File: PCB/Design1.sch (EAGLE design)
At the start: 23 parts, among them J1 FTDI_DEVICE, U1 ATMEGA2560AU

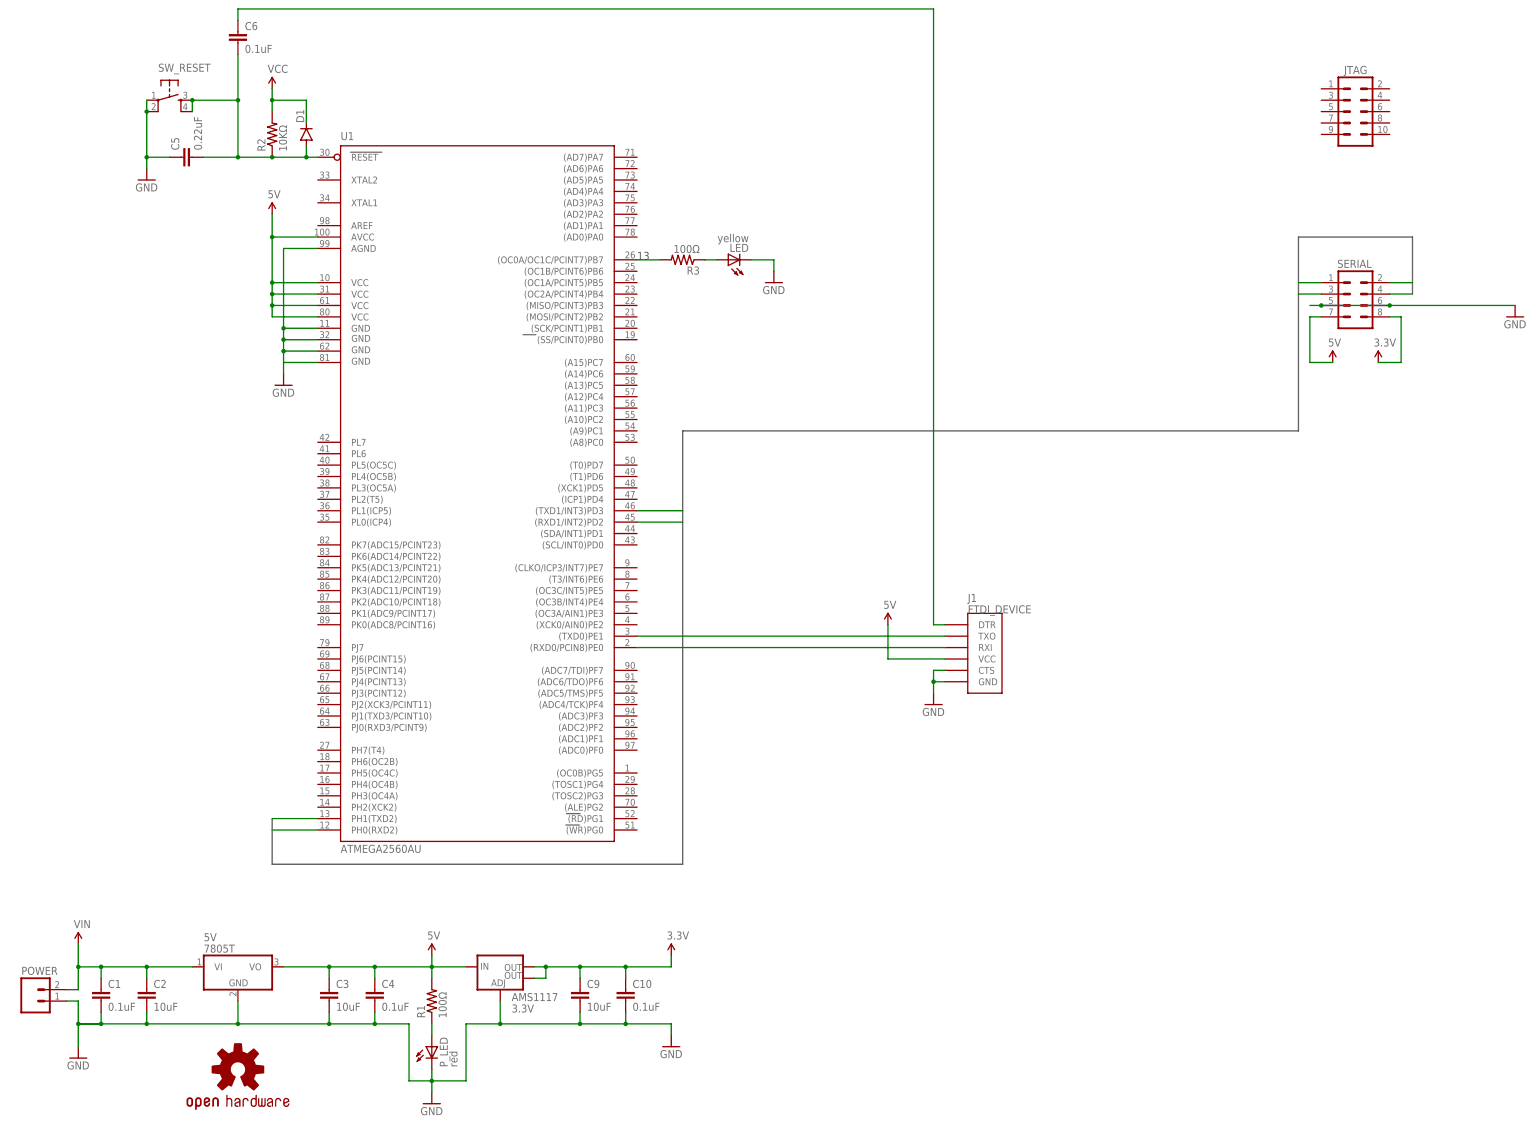
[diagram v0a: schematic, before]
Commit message: Update new Schematic
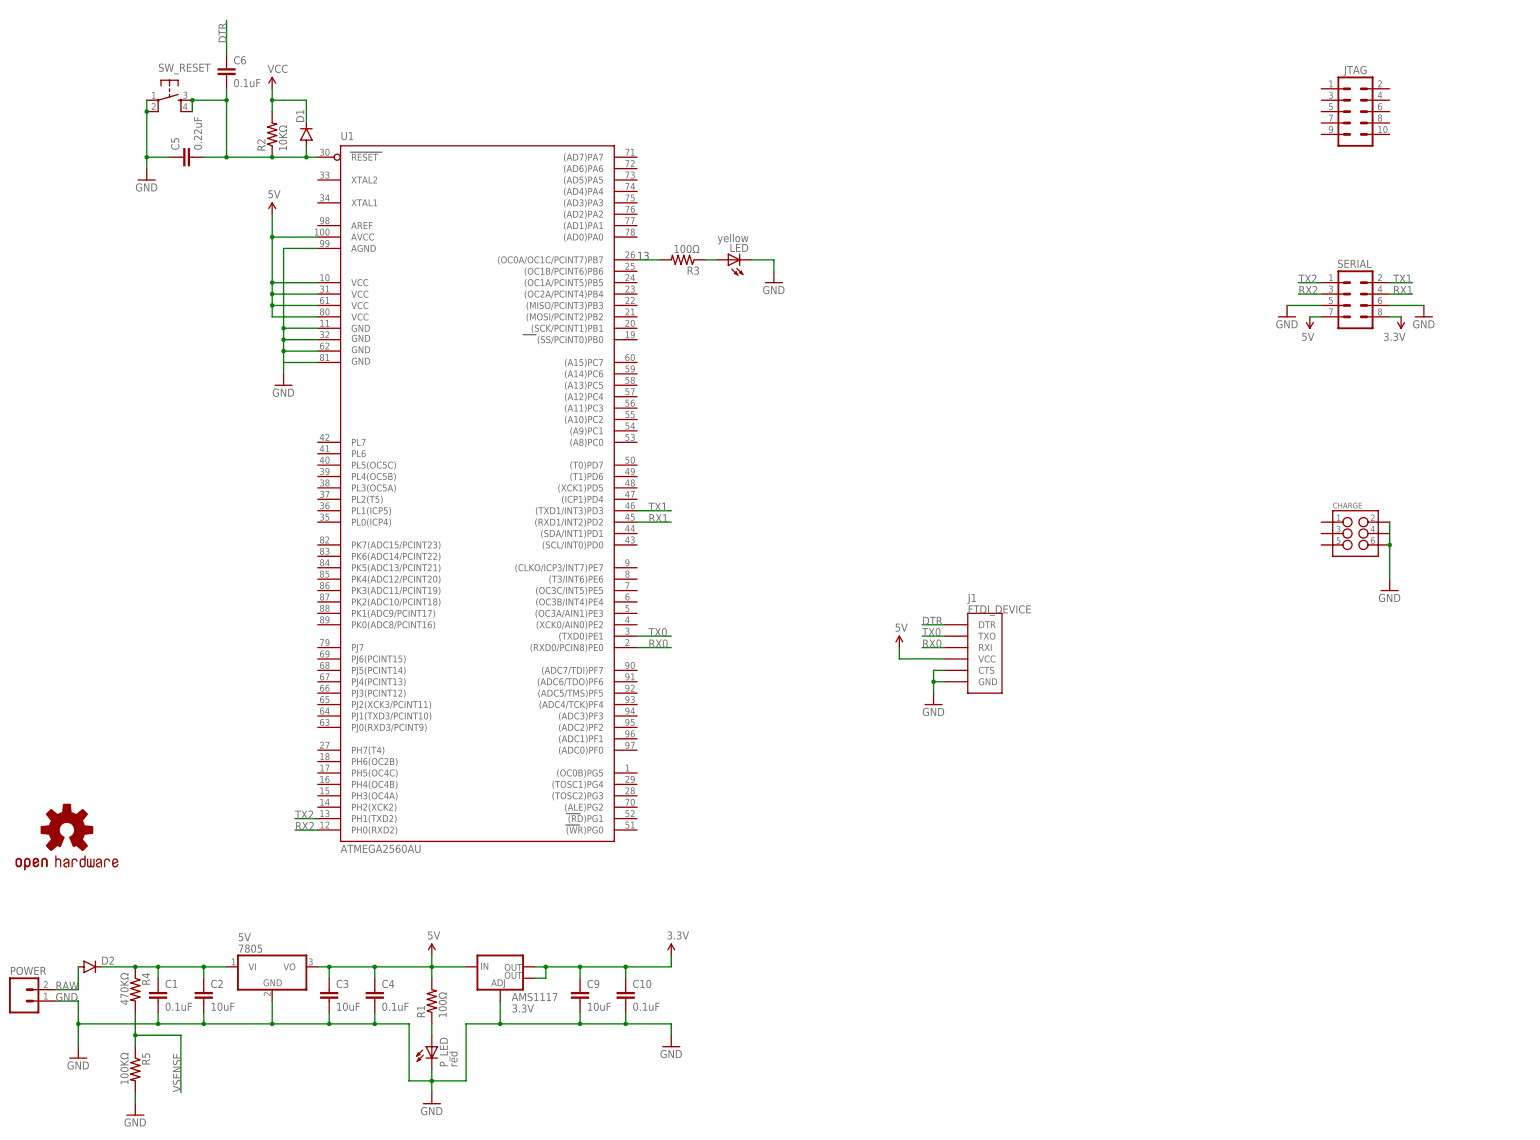
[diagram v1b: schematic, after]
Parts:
- added CHARGE: (no value), SparkFun-Connectors:M03X2FEMALE
- added D2: (no value), SparkFun-DiscreteSemi:DIODESMA-ALT
- added R4: 470KΩ, SparkFun-Resistors:RESISTOR1206
- added R5: 100KΩ, SparkFun-Resistors:RESISTOR1206
- 5V: value 7805T -> 7805
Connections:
- net SERIAL0 renamed TX1
- net SERIAL1 renamed RX1
- net SERIAL2 renamed TX2
- net SERIAL3 renamed RX2
- new net RAW: D2.A, POWER.2
- new net VSENSE: R4.2, R5.1
- net GND: now also CHARGE.2, CHARGE.6, R5.2
- net VIN: now also D2.C, R4.1; no longer POWER.2
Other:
- note added: "Power Source Mgmt"
- moved on the sheet: 5V, C1, C2, C6, POWER

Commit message: last nights' Schematic updates
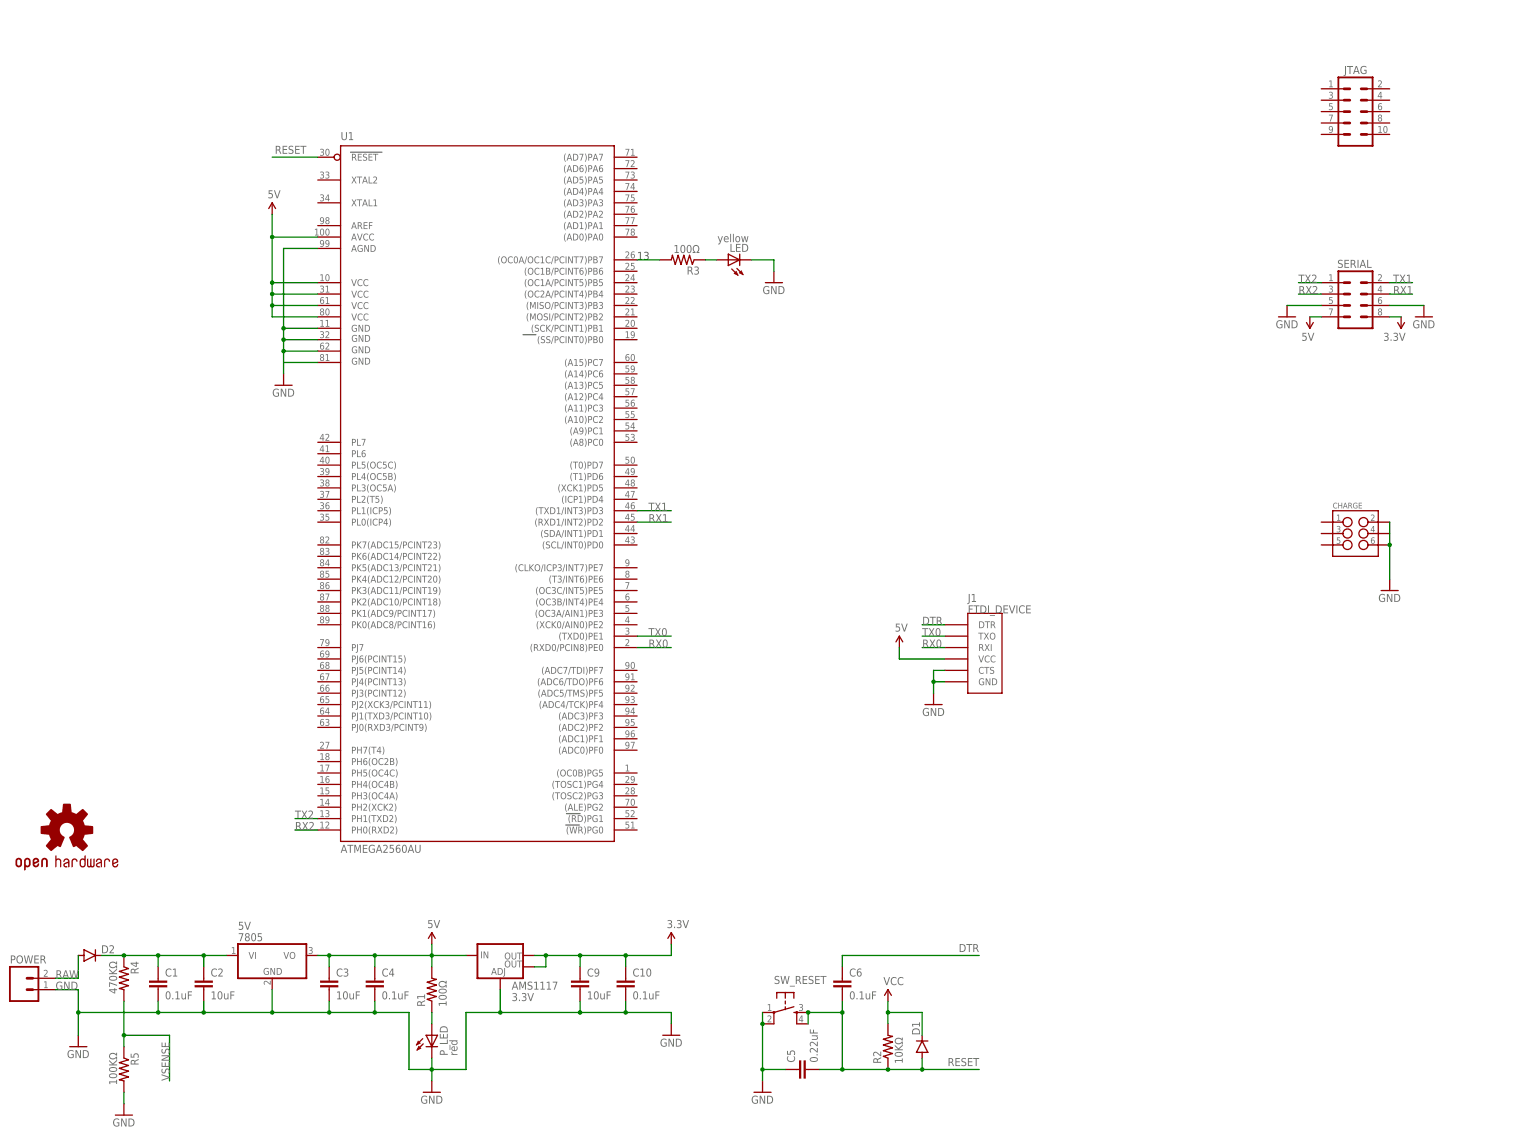
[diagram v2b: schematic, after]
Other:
- note added: "Reset circuitry"
- moved on the sheet: 5V, AMS1117, C1, C10, C2, C3, C4, C5, C6, C9, D1, D2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
